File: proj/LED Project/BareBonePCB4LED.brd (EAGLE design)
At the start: 160 x 100 mm, 13 parts, among them J3 AVR_SPI_PROG_3X2NS, Y1 16MHz

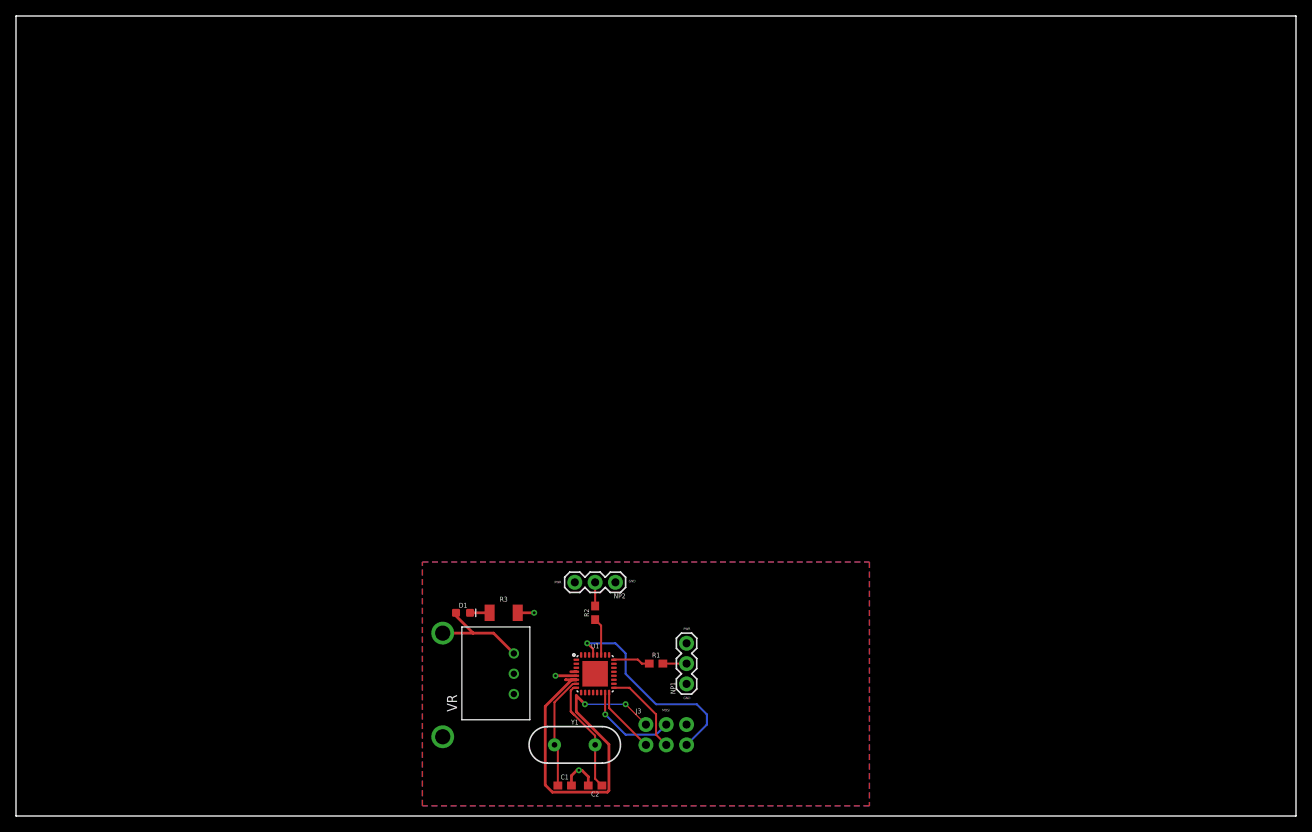
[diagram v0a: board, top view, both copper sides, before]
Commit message: fixes
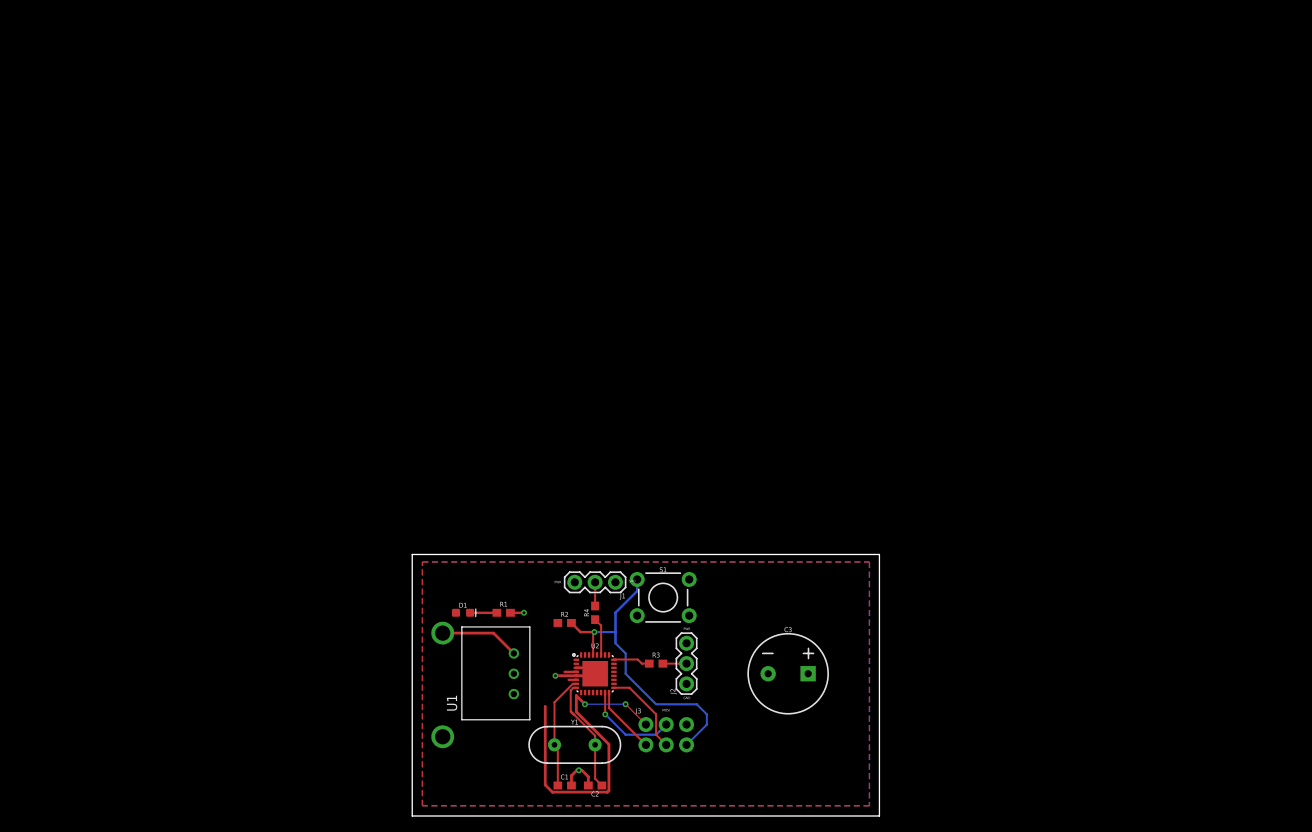
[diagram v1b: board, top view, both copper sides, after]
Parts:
- removed VR: R-78E5.0-1.0, SparkFun-IC-Power:DC-DC_CONVERTER_78XX
- added C3: 1mF, SparkFun-Capacitors:CPOL-RADIAL-5MM-10MM
- added R4: 400, SparkFun-Resistors:0603
- added S1: MOMENTARY-SWITCH-SPST-PTH-6.0MM-KIT, SparkFun-Switches:TACTILE_SWITCH_PTH_6.0MM_KIT
- added U2: (no value), SparkFun-IC-Microcontroller:MLF32-PAD
- R1: value 470 -> 83
- R2: value 470 -> 10k
- R3: value 500 -> 400; device SparkFun-Resistors:1210 -> SparkFun-Resistors:0603
- U1: value (none) -> R-78E5.0-1.0; device SparkFun-IC-Microcontroller:MLF32-PAD -> SparkFun-IC-Power:DC-DC_CONVERTER_78XX
- moved R1 20.1 mm to (61.0, 25.4)
- moved R3 20.1 mm to (80.0, 19.1)
- moved U1 10.2 mm to (62.2, 17.8), turned to 90 degrees
- moved R2 4.02 mm to (68.6, 24.1), turned to 0 degrees
- renumbered BAT to BT1, NP1 to J2, NP2 to J1
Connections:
- removed net N$11: C1.1, U1.7, Y1.1
- removed net N$12: C2.1, U1.8, Y1.2
- removed net N$2: J2.2, R1.2
- removed net N$5: J1.2, R2.2
- removed net N$8: R2.1, U1.27
- new net DATA: R4.1, U2.27
- new net DATA1: J2.2, R3.2
- new net DATA2: J1.2, R4.2
- new net XTAL1: C1.1, U2.7, Y1.1
- new net XTAL2: C2.1, U2.8, Y1.2
- net 9V: now also U1.VOUT; no longer D1.A, VR.VOUT
- net GND: now also C3.-, R1.2, S1.3, U1.GND, U2.3, U2.5, U2.PAD; no longer R3.2, U1.3, U1.5, VR.GND
- net MISO: now also U2.16; no longer U1.16
- net MOSI: now also U2.15; no longer U1.15
- net N$10: now also R1.1; no longer R3.1
- net N$7: now also R3.1, U2.24; no longer R1.1, U1.24
- net RST: now also R2.2, S1.1, U2.29; no longer U1.29
- net RX: now also U2.30; no longer U1.30
- net SCK: now also U2.17; no longer U1.17
- net TX: now also U2.31; no longer U1.31
- net VCC: now also C3.+, D1.A, R2.1, U1.VIN, U2.18, U2.4, U2.6; no longer U1.4, U1.6, VR.VIN
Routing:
- net XTAL2: track 0.00 -> 15.0 mm
- net N$12: track 15.0 -> 0.00 mm
- net XTAL1: track 0.00 -> 14.3 mm
- net N$11: track 14.3 -> 0.00 mm
- net RST: track 26.8 -> 39.8 mm
- net VCC: track 50.0 -> 44.4 mm
- net GND: track 9.72 -> 14.5 mm
- net N$8: track 4.73 -> 0.00 mm
- net DATA: track 0.00 -> 4.73 mm
- net 9V: track 13.4 -> 9.94 mm
- net N$5: track 2.96 -> 0.00 mm
- net DATA2: track 0.00 -> 2.96 mm
- net N$2: track 2.96 -> 0.00 mm
- net DATA1: track 0.00 -> 2.96 mm
- net N$10: track 2.45 -> 3.35 mm
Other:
- board size 160 x 100 mm -> 58.4 x 32.7 mm
